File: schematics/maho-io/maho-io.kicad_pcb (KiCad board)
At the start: 2 copper layers, 170 x 100 mm, 60 parts, among them J1 PWR, J2 V2, J3 V1

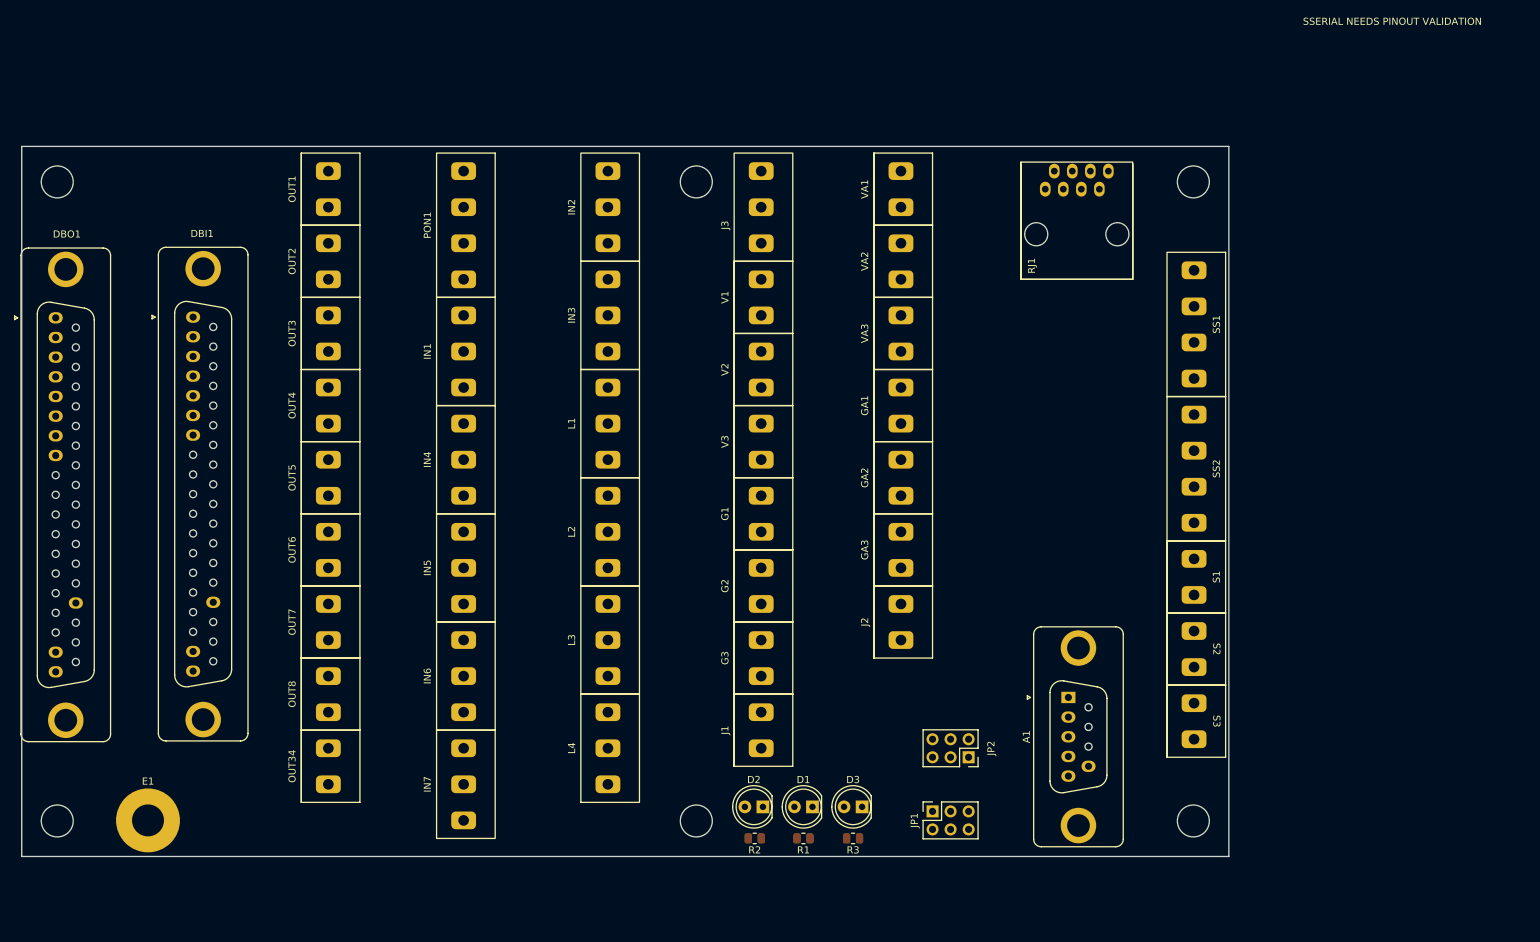
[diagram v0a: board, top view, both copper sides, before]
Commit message: board
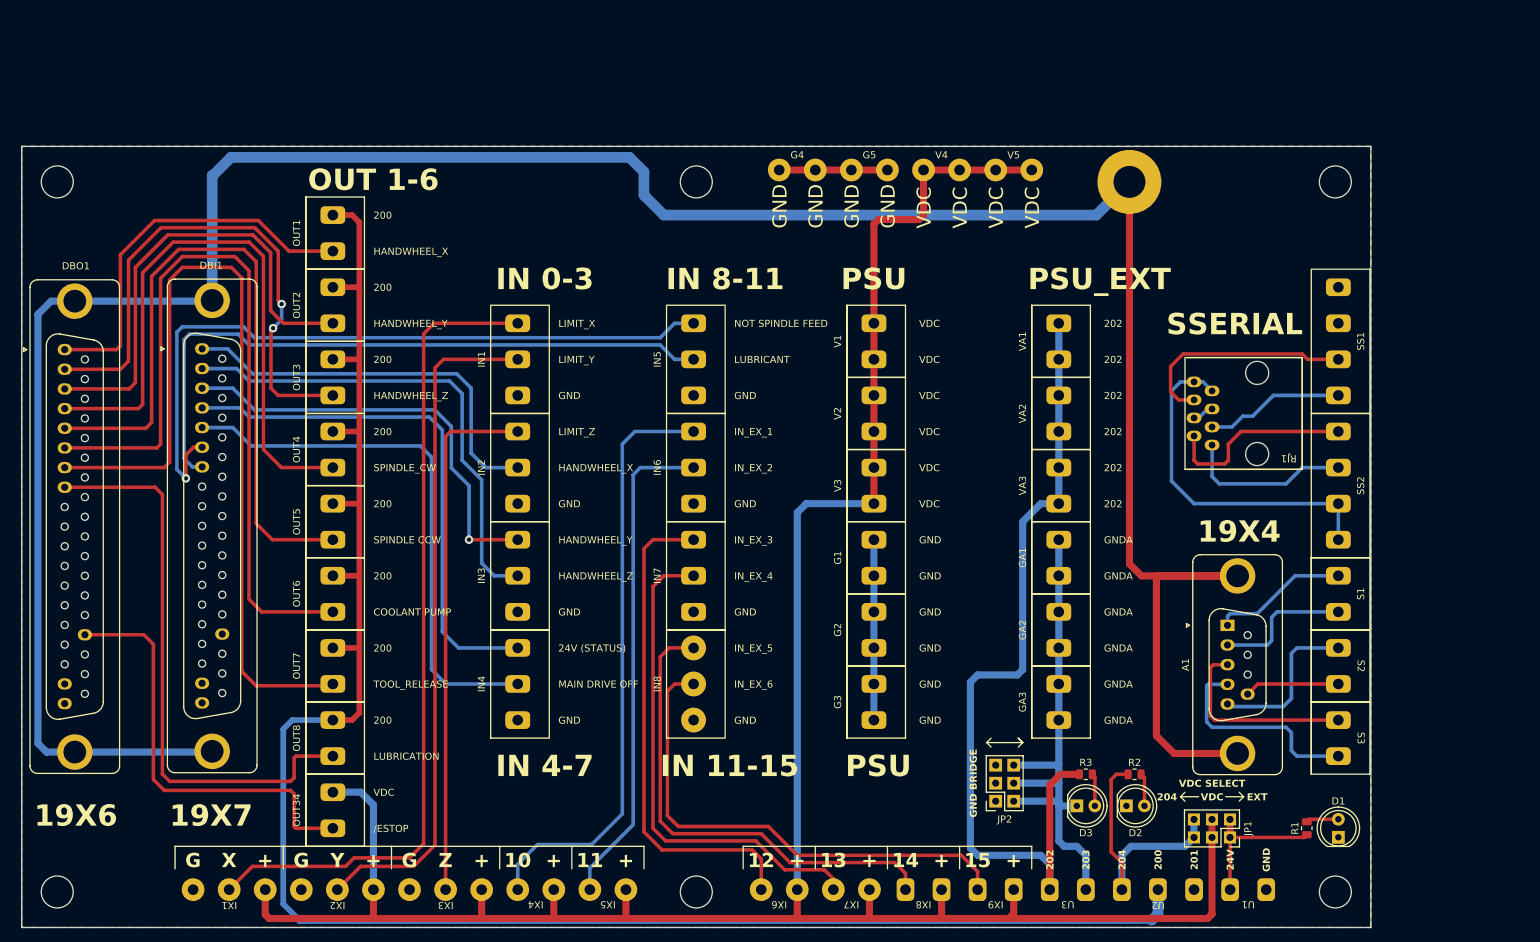
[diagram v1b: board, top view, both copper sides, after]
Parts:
- removed J1: PWR, XY2500V-C(5.08)-2P:XY2500V-C(5.08)-2P
- removed J2: V2, XY2500V-C(5.08)-2P:XY2500V-C(5.08)-2P
- removed J3: V1, XY2500V-C(5.08)-3P:XY2500V-C(5.08)-3P
- removed L1, L2, L3, L4: LIM, XY2500V-C(5.08)-3P:XY2500V-C(5.08)-3P
- removed PON1: POWER_ON_SWITCHES, XY2500V-C(5.08)-4P:XY2500V-C(5.08)-4P
- added G4: XY2500R-C(5.08)-2P, XY2500R-C(5.08)-2P:XY2500R-C(5.08)-2P, F.Cu at (181.3, 38.4)
- added G5: XY2500R-C(5.08)-2P, XY2500R-C(5.08)-2P:XY2500R-C(5.08)-2P, F.Cu at (191.5, 38.4)
- added IN8: IN, XY2500V-C(5.08)-3P:XY2500V-C(5.08)-3P, F.Cu at (166.7, 110.7)
- added IX1: XY2500R-C(5.08)-3P, XY2500R-C(5.08)-3P:XY2500R-C(5.08)-3P, F.Cu at (101.3, 139.7)
- added IX2: XY2500R-C(5.08)-3P, XY2500R-C(5.08)-3P:XY2500R-C(5.08)-3P, F.Cu at (116.5, 139.7)
- added IX3: XY2500R-C(5.08)-3P, XY2500R-C(5.08)-3P:XY2500R-C(5.08)-3P, F.Cu at (131.8, 139.7)
- added IX4: XY2500R-C(5.08)-2P, XY2500R-C(5.08)-2P:XY2500R-C(5.08)-2P, F.Cu at (144.5, 139.7)
- added IX5: XY2500R-C(5.08)-2P, XY2500R-C(5.08)-2P:XY2500R-C(5.08)-2P, F.Cu at (154.6, 139.7)
- added IX6: XY2500R-C(5.08)-2P, XY2500R-C(5.08)-2P:XY2500R-C(5.08)-2P, F.Cu at (178.8, 139.7)
- added IX7: XY2500R-C(5.08)-2P, XY2500R-C(5.08)-2P:XY2500R-C(5.08)-2P, F.Cu at (188.9, 139.7)
- added IX8: XY2500R-C(5.08)-2P, XY2500R-C(5.08)-2P:XY2500R-C(5.08)-2P, F.Cu at (199.1, 139.7)
- added IX9: XY2500R-C(5.08)-2P, XY2500R-C(5.08)-2P:XY2500R-C(5.08)-2P, F.Cu at (209.2, 139.7)
- added U1: XY2500R-C(5.08)-2P, XY2500R-C(5.08)-2P:XY2500R-C(5.08)-2P, F.Cu at (244.8, 139.7)
- added U2: XY2500R-C(5.08)-3P, XY2500R-C(5.08)-3P:XY2500R-C(5.08)-3P, F.Cu at (232.1, 139.7)
- added U3: XY2500R-C(5.08)-2P, XY2500R-C(5.08)-2P:XY2500R-C(5.08)-2P, F.Cu at (219.4, 139.7)
- added V4: XY2500R-C(5.08)-2P, XY2500R-C(5.08)-2P:XY2500R-C(5.08)-2P, F.Cu at (201.6, 38.4)
- added V5: XY2500R-C(5.08)-2P, XY2500R-C(5.08)-2P:XY2500R-C(5.08)-2P, F.Cu at (211.8, 38.4)
- IN1: value IN1 -> IN
- IN2: value IN2 -> IN
- IN3: value IN3 -> IN
- IN4: value IN4 -> IN
- IN5: value IN5 -> IN
- IN6: value IN6 -> IN
- IN7: value IN7 -> IN
- OUT1: value OUT1 -> OUT
- OUT2: value OUT2 -> OUT
- OUT3: value OUT3 -> OUT
- OUT34: value OUT34 -> OUT
- OUT4: value OUT4 -> OUT
- OUT5: value OUT5 -> OUT
- OUT6: value OUT6 -> OUT
- OUT7: value OUT7 -> OUT
- OUT8: value OUT8 -> OUT
- moved E1 164.9 mm to (228.1, 40.0)
- moved D1 74.2 mm to (257.5, 132.3), turned to 90 degrees
- moved R1 70.9 mm to (253.1, 131.1), turned to 90 degrees
- moved R2 54.3 mm to (228.8, 123.5), turned to 0 degrees
- moved D2 51.2 mm to (227.7, 127.9), turned to 0 degrees
- moved IN5 43.7 mm to (166.7, 65.0)
- moved IN7 43.7 mm to (166.7, 95.5)
- moved IN6 43.7 mm to (166.7, 80.3)
- moved JP1 42.1 mm to (242.3, 132.3), turned to -90 degrees
- moved IN2 38.8 mm to (141.9, 80.3)
- moved IN3 38.8 mm to (141.9, 95.5)
- moved RJ1 35.8 mm to (246.1, 72.6), turned to 90 degrees
- moved R3 34.0 mm to (221.9, 123.5), turned to 0 degrees
- moved IN4 32.5 mm to (141.9, 110.7)
- moved GA2 30.9 mm to (218.1, 103.1)
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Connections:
- A1 pad 0: unconnected-(A1-PAD-Pad0) -> Earth
- DBI1 pad 2: /19X7_HANDWHEEL_Y -> /19X7_HANDWHEEL_Z
- DBI1 pad 3: /19X7_HANDWHEEL_Z -> /19X7_HANDWHEEL_Y
- IN1 pad 1: /EXTERNAL_ESTOP -> /LIMIT_X
- IN1 pad 2: /POWER_SWITCH -> /LIMIT_Υ
- IN2 pad 1: /LIMIT_X -> /LIMIT_Ζ
- IN2 pad 2: /LIMIT_Υ -> /19X7_HANDWHEEL_X
- IN3 pad 1: /LIMIT_Ζ -> /19X7_HANDWHEEL_Y
- IN3 pad 2: /LIMIT_Α -> /19X7_HANDWHEEL_Z
- IN4 pad 1: /19X7_HANDWHEEL_X -> /19X7_24V
- IN4 pad 2: /19X7_HANDWHEEL_Y -> /19X7_MAIN_DRIVE_OFF
- IN5 pad 1: /19X7_HANDWHEEL_Z -> /19X7_NOT_SPINDLE_FEED
- IN5 pad 2: /19X7_24V -> /19X7_LUBRICANT
- IN6 pad 1: /19X7_MAIN_DRIVE_OFF -> /IN10
- IN6 pad 2: /19X7_NOT_SPINDLE_FEED -> /IN11
- IN7 pad 1: /19X7_LUBRICANT -> /IN12
- IN7 pad 2: unconnected-(IN7-Pad2) -> /IN13
- SS1 pad 1: /SS_5VP -> GND
- SS1 pad 2: /SS_5VP -> GND
- SS2 pad 3: GND -> /SS_5VP
- SS2 pad 4: GND -> /SS_5VP
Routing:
- net Earth: track 0.00 -> 382.1 mm
- net VDC: track 0.00 -> 334.9 mm
- net /200_NORMAL: track 0.00 -> 260.1 mm
- net /TOOL_RELEASE: track 0.00 -> 121.4 mm
- net /202_24V: track 0.00 -> 119.0 mm
- net /LIMIT_X: track 0.00 -> 115.7 mm
- net /COOLANT_PUMP: track 0.00 -> 110.4 mm
- net /19X7_NOT_SPINDLE_FEED: track 0.00 -> 101.7 mm, vias 0 -> 1
- net /SPINDLE_CCW: track 0.00 -> 98.8 mm
- net /LIMIT_Υ: track 0.00 -> 95.7 mm
- net /19X7_LUBRICANT: track 0.00 -> 93.3 mm
- net /SPINDLE_CW: track 0.00 -> 87.4 mm
- net /IN10: track 0.00 -> 84.1 mm
- net /CENTRAL_LUBRICATION: track 0.00 -> 81.1 mm
- net /19X6_HANDWHEEL_Z: track 0.00 -> 77.3 mm, vias 0 -> 2
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- added copper zone on B.Cu, net GND
- added copper zone on F.Cu, net GND
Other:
- board size 170 x 100 mm -> 190 x 110 mm
- board text added: "+"
- board text added: "/ESTOP"
- board text added: "10"
- board text added: "11"
- board text added: "12"
- board text added: "13"
- board text added: "14"
- board text added: "15"
- board text added: "19X4"
- board text added: "19X6"
- board text added: "19X7"
- board text added: "200"
- board text added: "201"
- board text added: "202"
- board text added: "203"
- board text added: "204"
- board text added: "24V"
- board text added: "24V (STATUS)"
- board text added: "COOLANT PUMP"
- board text added: "EXT"
- board text added: "G"
- board text added: "GND"
- board text added: "GND BRIDGE"
- board text added: "GNDA"
- board text added: "HANDWHEEL_X"
- board text added: "HANDWHEEL_Y"
- board text added: "HANDWHEEL_Z"
- board text added: "IN 0-3"
- board text added: "IN 11-15"
- board text added: "IN 4-7"
- board text added: "IN 8-11"
- board text added: "IN_EX_1"
- board text added: "IN_EX_2"
- board text added: "IN_EX_3"
- board text added: "IN_EX_4"
- board text added: "IN_EX_5"
- board text added: "IN_EX_6"
- board text added: "LIMIT_X"
- board text added: "LIMIT_Y"
- board text added: "LIMIT_Z"
- board text added: "LUBRICANT"
- board text added: "LUBRICATION"
- board text added: "MAIN DRIVE OFF"
- board text added: "NOT SPINDLE FEED"
- board text added: "OUT 1-6"
- board text added: "PSU"
- board text added: "PSU_EXT"
- board text added: "SPINDLE CCW"
- board text added: "SPINDLE_CW"
- board text added: "SSERIAL"
- board text added: "TOOL_RELEASE"
- board text added: "VDC"
- board text added: "VDC SELECT"
- board text added: "X"
- board text added: "Y"
- board text added: "Z"
- board text removed: "SSERIAL NEEDS PINOUT VALIDATION"
